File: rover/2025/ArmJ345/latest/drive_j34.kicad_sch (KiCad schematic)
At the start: 18 parts, among them J10 JST-PH-S6B, J7 XT30PW-M, J8 XT30PW-M, J9 JST-PH-S6B, U8 IFX9201SGAUMA1, U9 IFX9201SGAUMA1

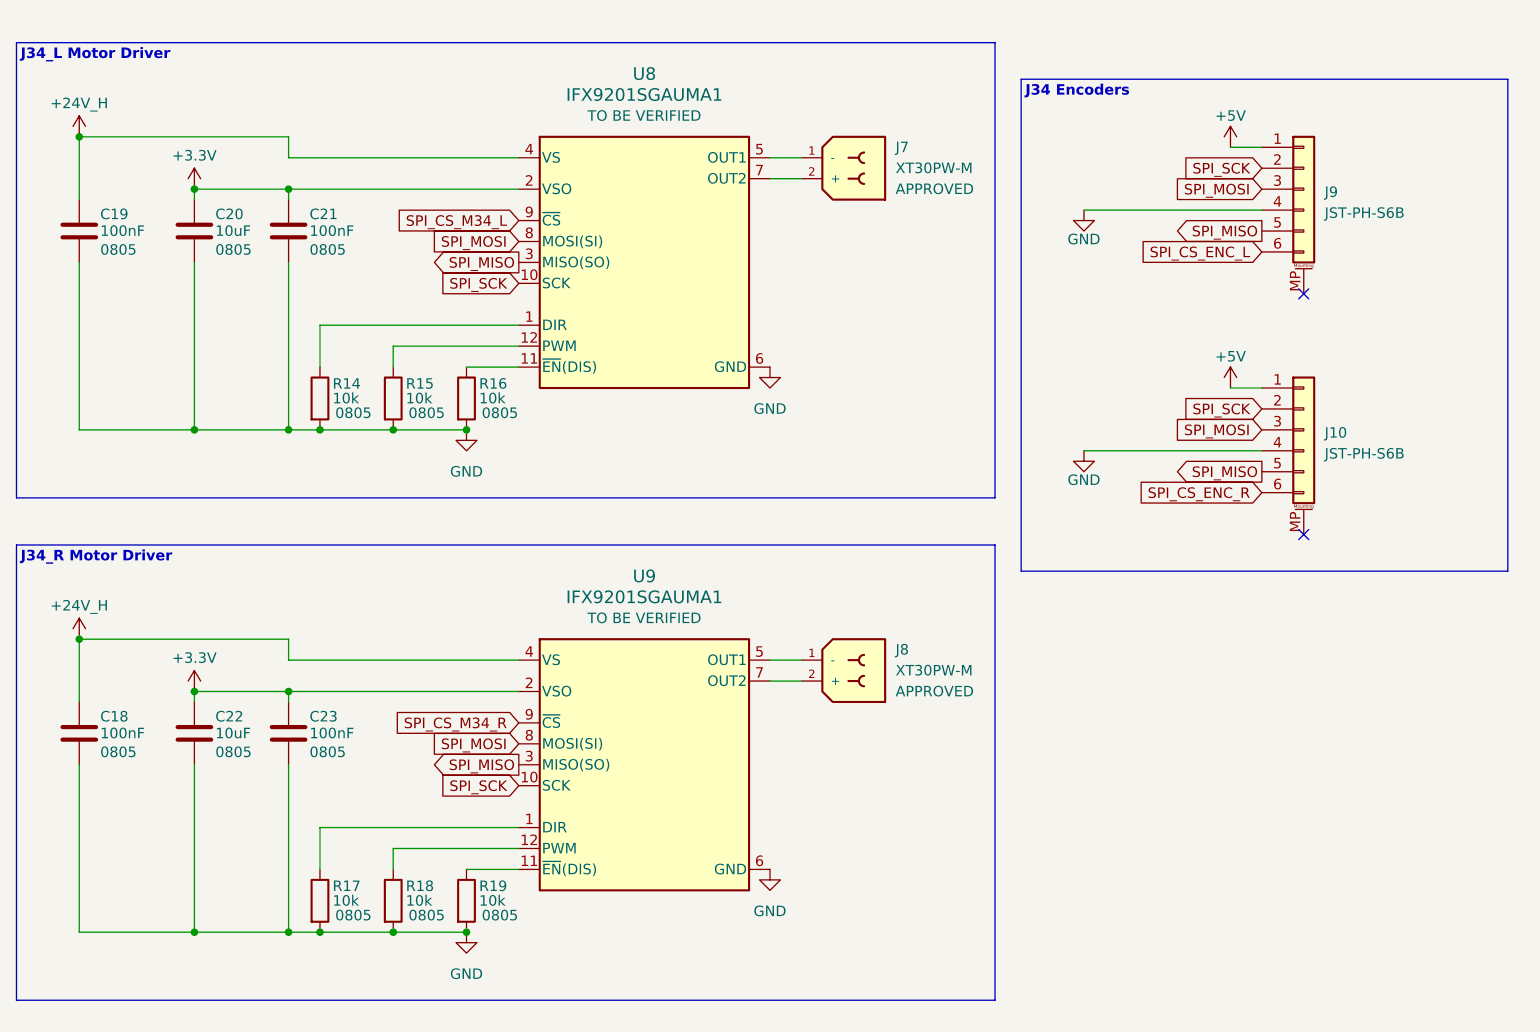
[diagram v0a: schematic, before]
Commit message: armj345 fixes
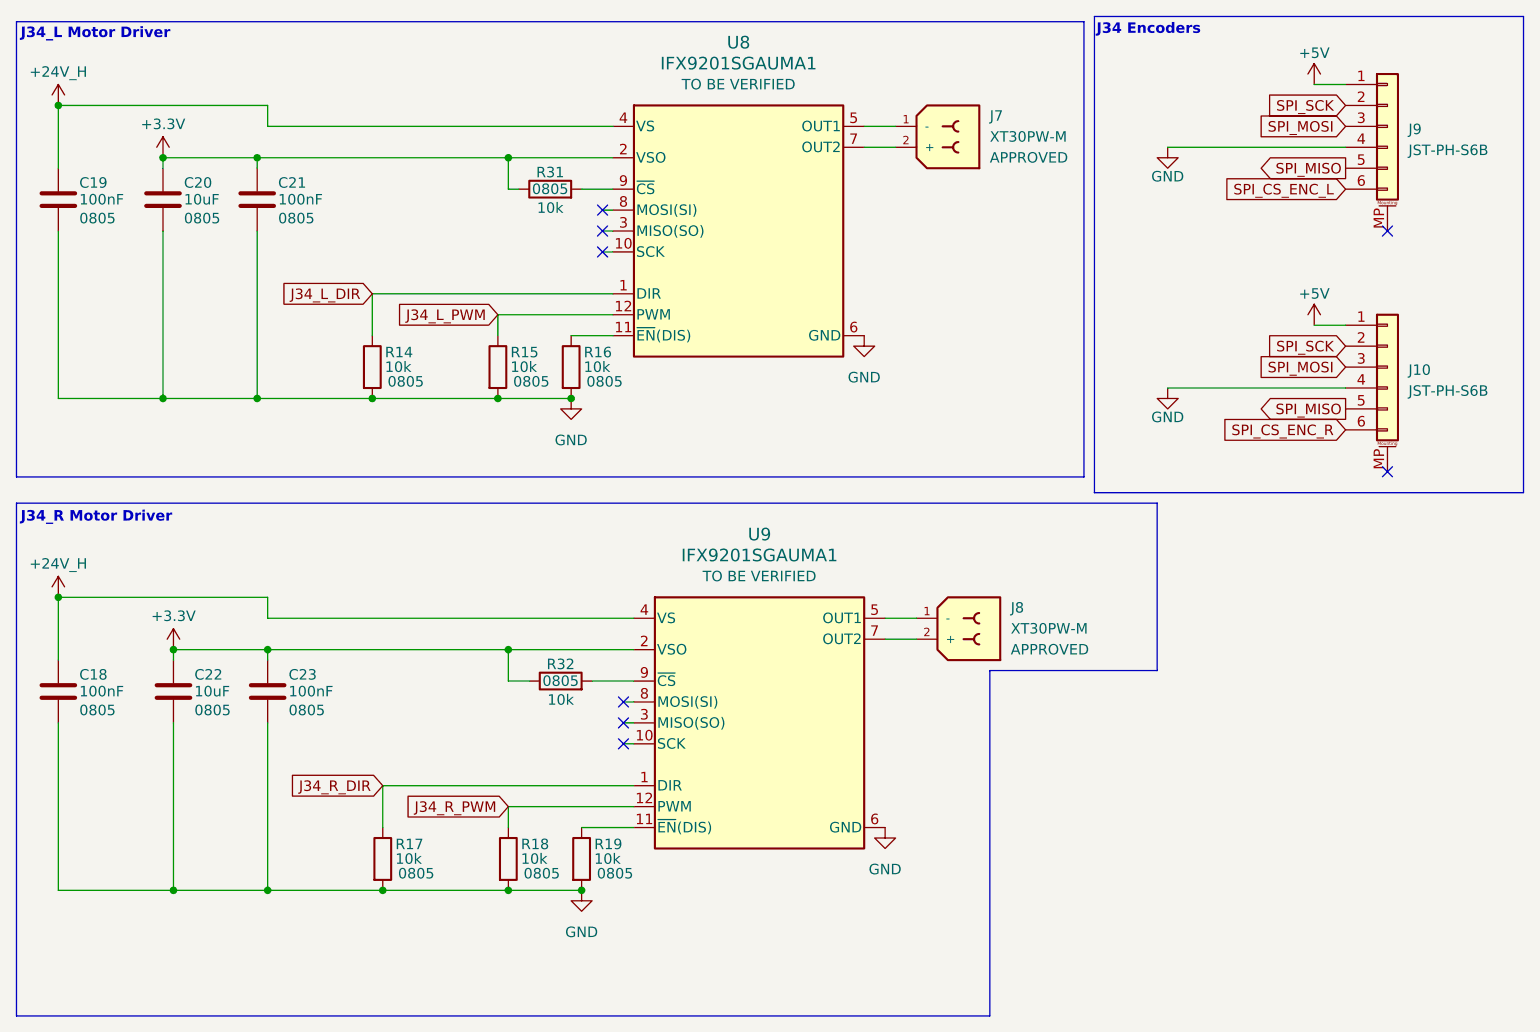
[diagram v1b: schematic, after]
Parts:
- added R31, R32: 10k, Resistor_SMD:R_0805_2012Metric_Pad1.20x1.40mm_HandSolder, symbol RoverLibrary:R_0805
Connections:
- net +3.3V: now also R31.1, R32.1
- net SPI_MISO: no longer U8.3 (MISO(SO)), U9.3 (MISO(SO))
- net SPI_MOSI: no longer U8.8 (MOSI(SI)), U9.8 (MOSI(SI))
- net SPI_SCK: no longer U8.10 (SCK), U9.10 (SCK)
- net J34_L_DIR: now reaches R14.1, U8.1 (DIR)
- net J34_L_PWM: now reaches R15.1, U8.12 (PWM)
- net J34_R_DIR: now reaches R17.1, U9.1 (DIR)
- net J34_R_PWM: now reaches R18.1, U9.12 (PWM)
- net SPI_CS_M34_L: no longer names the net of U8.9 (~{CS})
- net SPI_CS_M34_L: now also R31.2
- net SPI_CS_M34_R: no longer names the net of U9.9 (~{CS})
- net SPI_CS_M34_R: now also R32.2
- no-connect marks 2 -> 8
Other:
- moved on the sheet: C18, C19, C20, C21, C22, C23, J10, J7, J8, J9, R14, R15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
